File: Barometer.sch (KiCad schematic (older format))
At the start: 5 parts, among them U7 BMP280

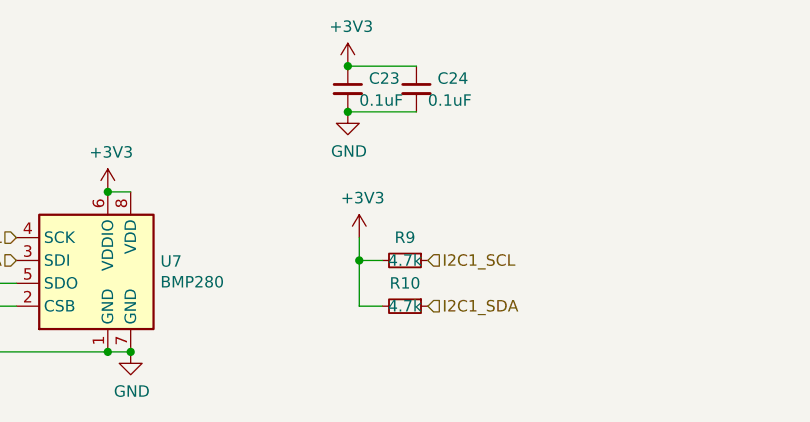
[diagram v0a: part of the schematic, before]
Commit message: Finished routing
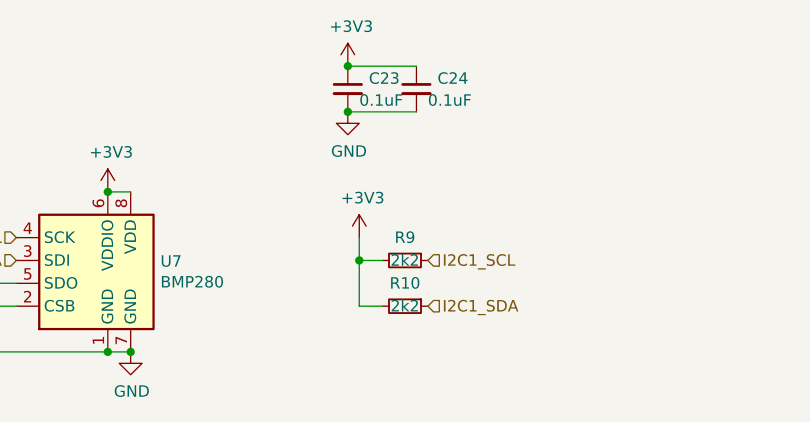
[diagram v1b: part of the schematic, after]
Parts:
- R10, R9: value 4.7k -> 2k2
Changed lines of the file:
@@
 P 8150 4650
 F 0 "R9" V 8050 4650 50  0000 C CNN
-F 1 "4.7k" V 8150 4650 50  0000 C CNN
+F 1 "2k2" V 8150 4650 50  0000 C CNN
 F 2 "Resistor_SMD:R_0402_1005Metric" H 8150 4650 50  0001 C CNN
 F 3 "~" H 8150 4650 50  0001 C CNN
@@
 P 8150 4850
 F 0 "R10" V 8050 4850 50  0000 C CNN
-F 1 "4.7k" V 8150 4850 50  0000 C CNN
+F 1 "2k2" V 8150 4850 50  0000 C CNN
 F 2 "Resistor_SMD:R_0402_1005Metric" H 8150 4850 50  0001 C CNN
 F 3 "~" H 8150 4850 50  0001 C CNN
